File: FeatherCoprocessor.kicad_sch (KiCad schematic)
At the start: 2 parts, among them J2 Conn_02x28_Odd_Even, U11 Adafruit_FeatherWing

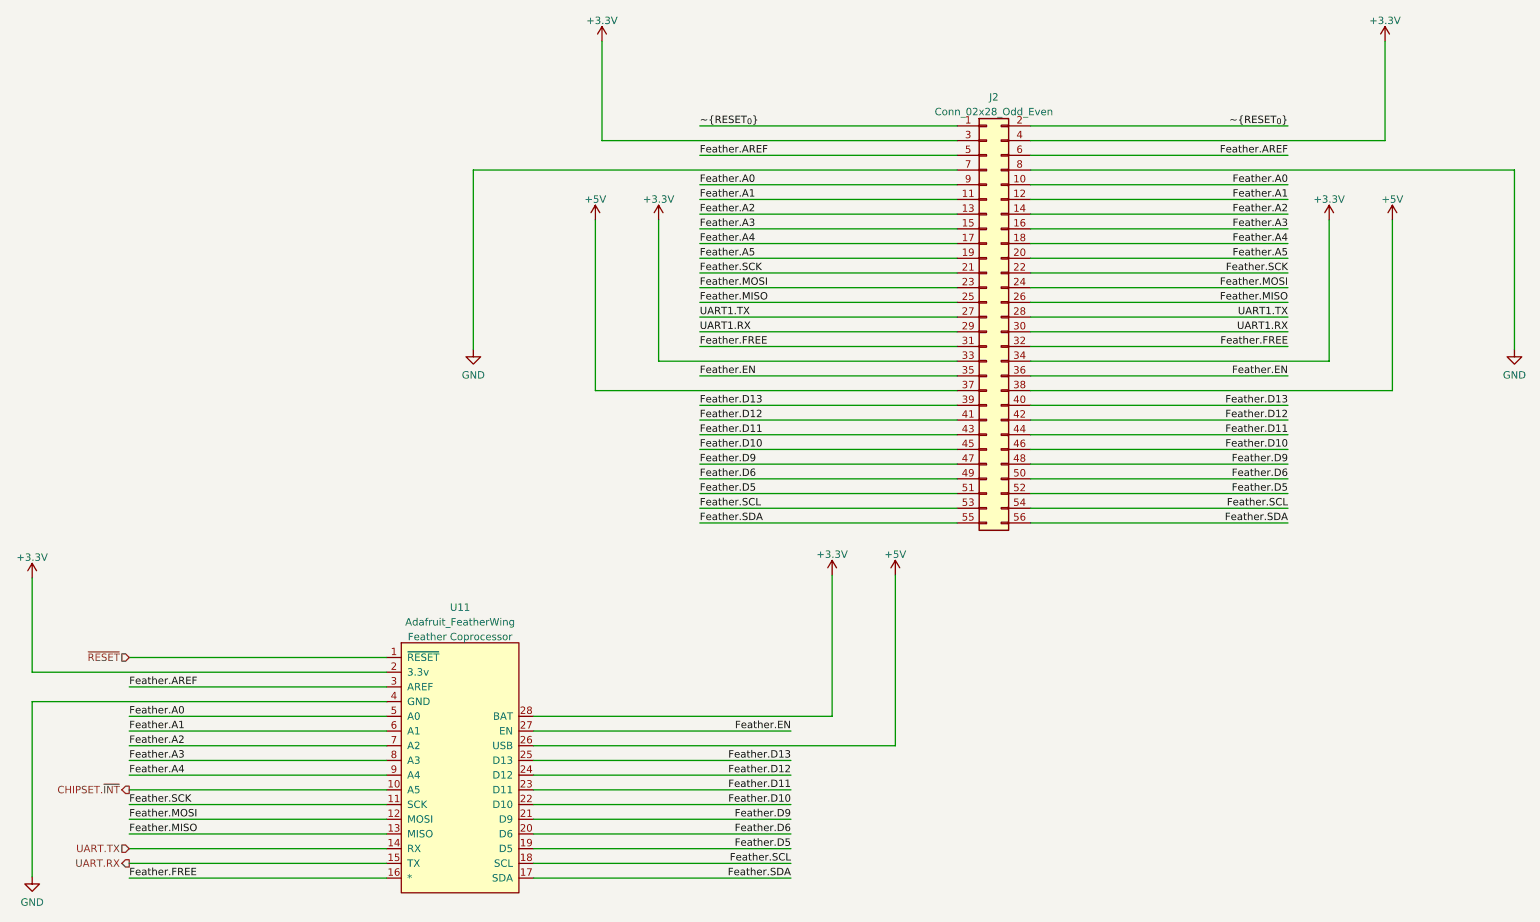
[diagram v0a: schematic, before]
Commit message: Only have one feather
Also came up with a good layout in the form of a "card" style that can
easily be moved around for the i960
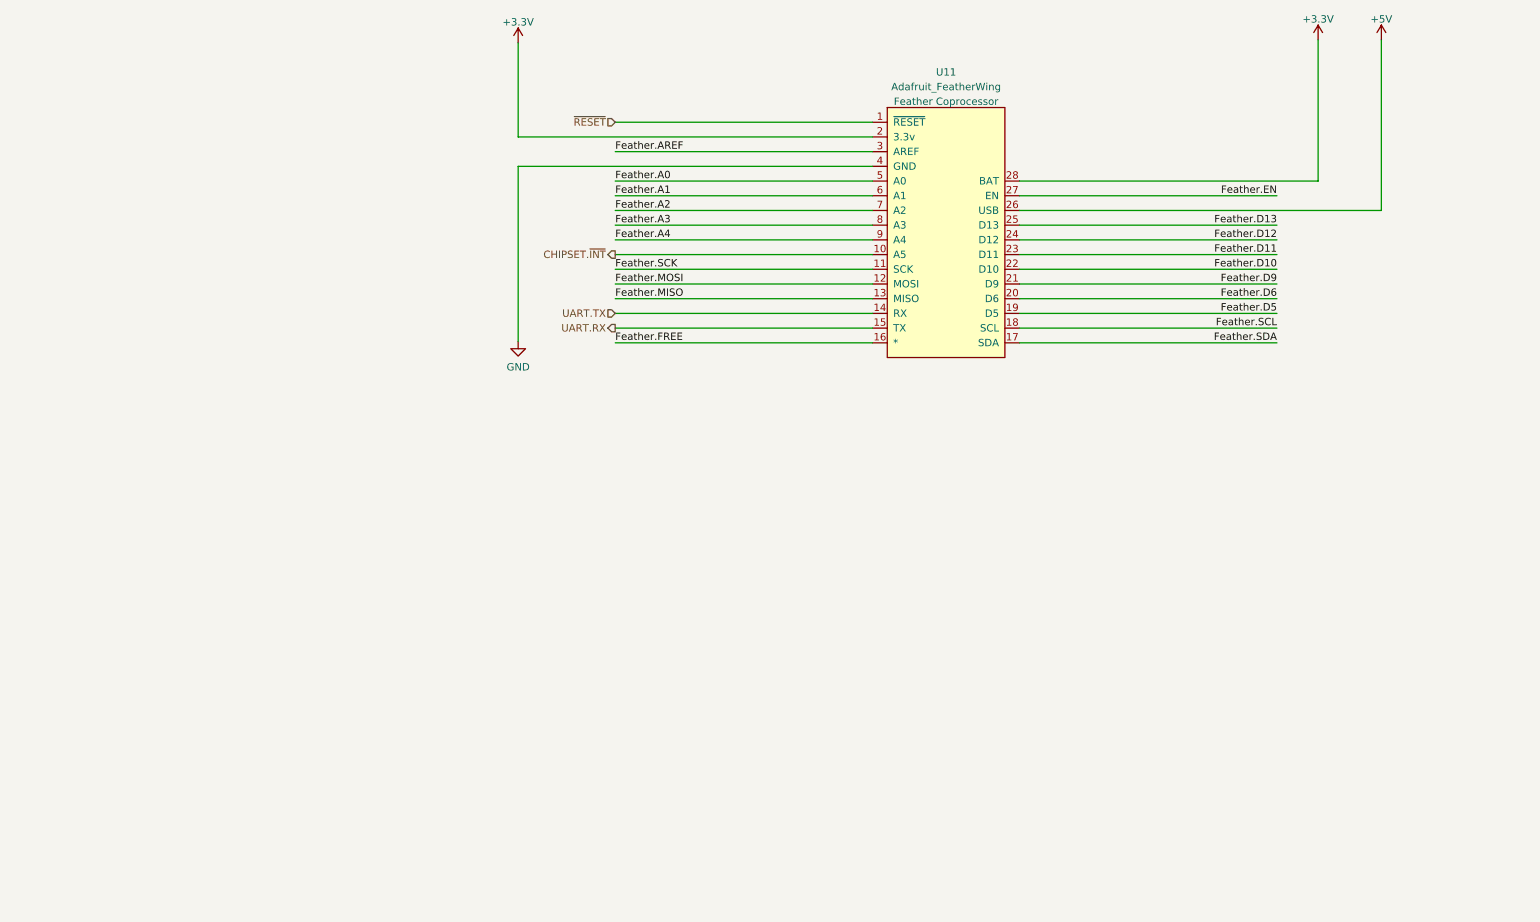
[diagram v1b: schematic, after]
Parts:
- removed J2: Conn_02x28_Odd_Even, Connector_PinHeader_2.54mm:PinHeader_2x28_P2.54mm_Vertical, symbol Connector_Generic:Conn_02x28_Odd_Even
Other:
- moved on the sheet: U11
